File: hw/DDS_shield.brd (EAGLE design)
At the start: 73.3 x 58.4 mm, 32 parts, among them K1 mode, U1 ARDUINOR3-BPLACE, X1 F-out, X2 Input

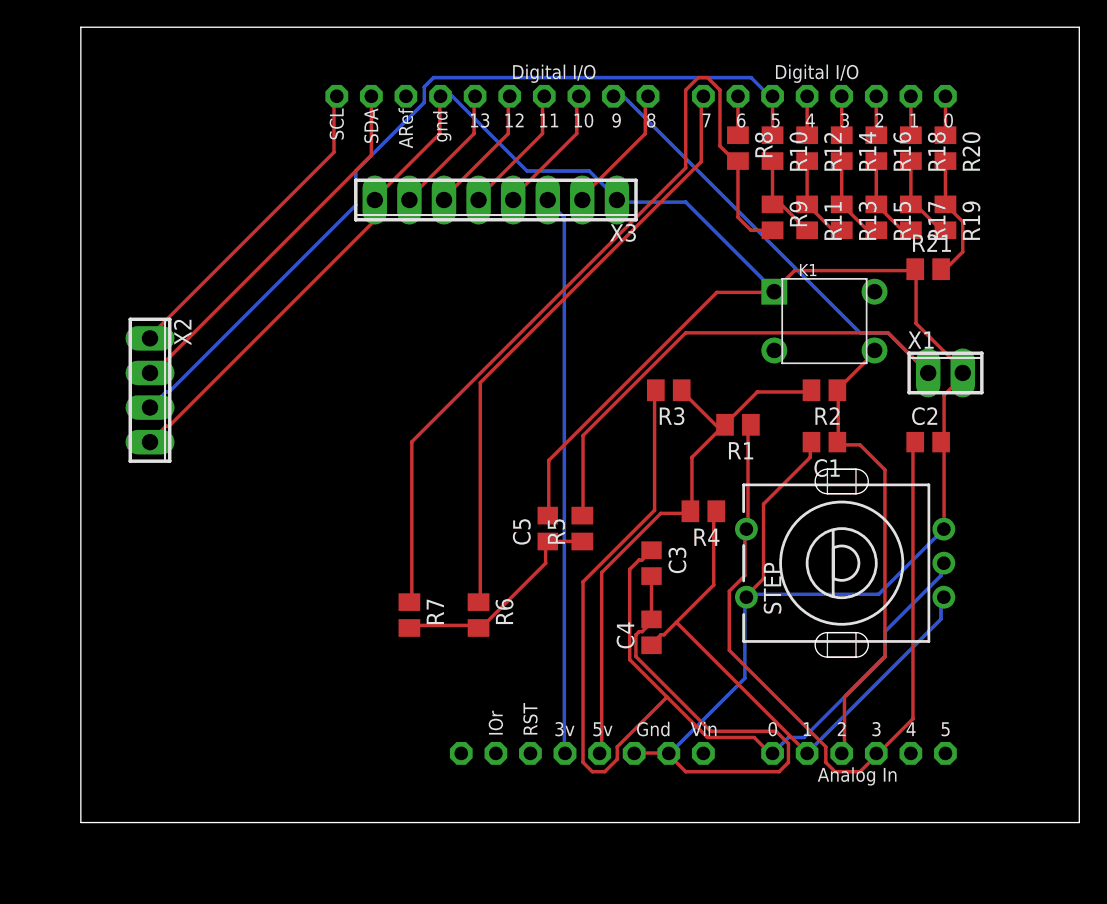
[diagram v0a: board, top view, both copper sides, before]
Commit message: final board
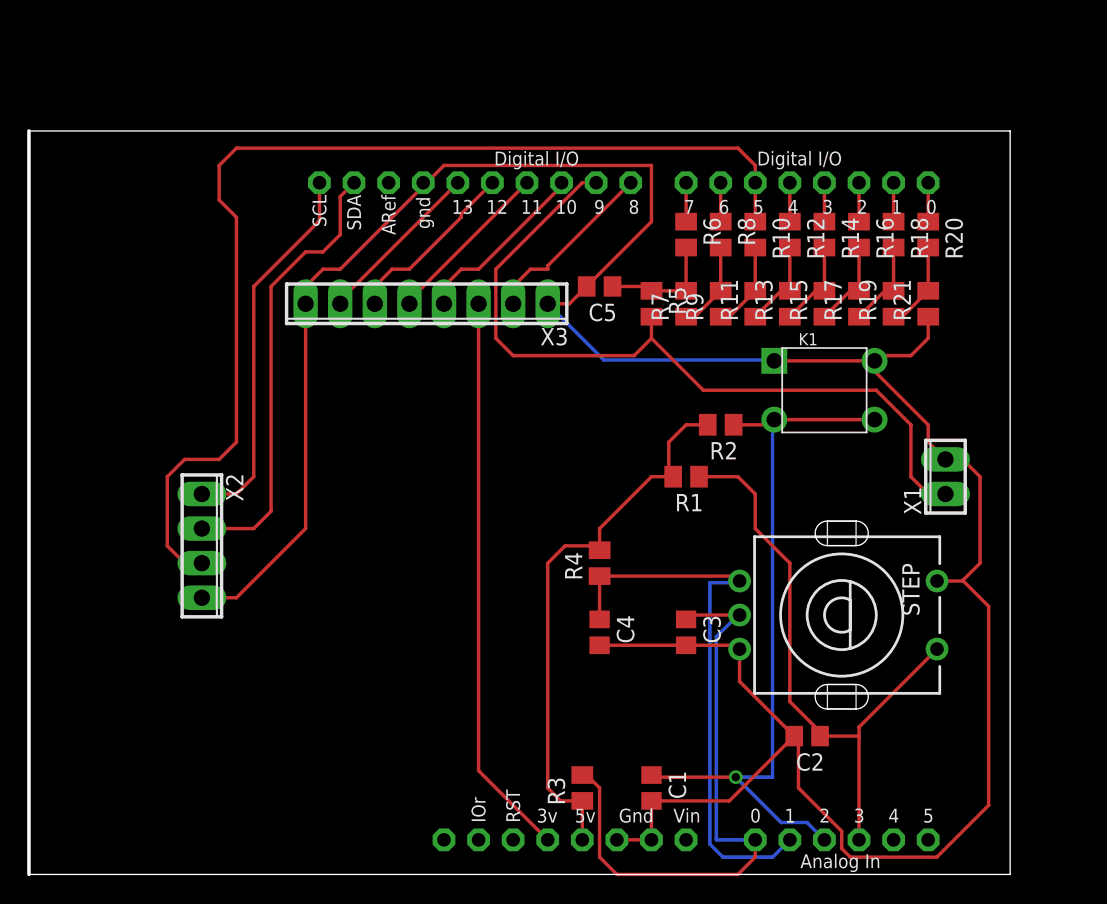
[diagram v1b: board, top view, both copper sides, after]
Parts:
- X3: value (none) -> screen
- moved R6 31.8 mm to (71.1, 47.0)
- moved R7 30.6 mm to (71.1, 41.9), turned to 90 degrees
- moved R3 29.9 mm to (63.5, 6.35), turned to 90 degrees
- moved C1 28.4 mm to (68.6, 6.35), turned to 270 degrees
- moved C2 23.3 mm to (80.0, 10.2), turned to 180 degrees
- moved C5 18.2 mm to (64.8, 43.2), turned to 180 degrees
- moved R5 17.3 mm to (68.6, 41.9), turned to 270 degrees
- moved X2 12.0 mm to (35.6, 24.1)
- moved X3 9.16 mm to (52.1, 41.9)
- moved R4 8.52 mm to (64.8, 22.9), turned to 90 degrees
- moved R2 8.03 mm to (73.7, 33.0)
- moved X1 7.62 mm to (90.2, 29.2), turned to 90 degrees
- moved R11 7.41 mm to (76.2, 41.9), turned to 90 degrees
- moved R13 7.41 mm to (78.7, 41.9), turned to 90 degrees
- moved R15 7.41 mm to (81.3, 41.9), turned to 90 degrees
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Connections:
- net GND: now also K1.4
- net N$1: now also K1.2
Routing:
- net N$14: track 62.3 -> 6.51 mm
- net N$8: track 44.1 -> 2.86 mm
- net N$5: track 80.9 -> 44.7 mm
- net N$1: track 34.6 -> 54.3 mm, vias 0 -> 1
- net N$10: track 61.3 -> 79.7 mm
- net N$2: track 57.2 -> 43.7 mm
- net N$6: track 67.1 -> 57.7 mm
- net N$7: track 16.4 -> 8.71 mm
- net N$24: track 27.3 -> 33.0 mm
- net N$25: track 23.6 -> 27.9 mm
- net N$23: track 9.93 -> 13.5 mm
- net N$29: track 9.74 -> 13.2 mm
- net N$27: track 9.83 -> 13.2 mm
- net N$22: track 9.31 -> 6.51 mm
- net N$30: track 9.70 -> 12.5 mm
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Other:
- board size 73.3 x 58.4 mm -> 72.1 x 54.6 mm
